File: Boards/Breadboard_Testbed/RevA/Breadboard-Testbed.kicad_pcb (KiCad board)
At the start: 2 copper layers, 85 x 56 mm, 12 parts, among them J1 main_conn_10, J10 Arduino-right, J12 Conn_02x12_Counter_Clockwise, J2 main_conn_12, J3 Conn_02x14_Odd_Even, J4 Conn_02x14_Odd_Even, J5 Conn_02x10_Counter_Clockwise, J6 Conn_02x14_Odd_Even, J7 Arduino-left, J8 Conn_02x10_Counter_Clockwise, J9 Conn_02x12_Counter_Clockwise

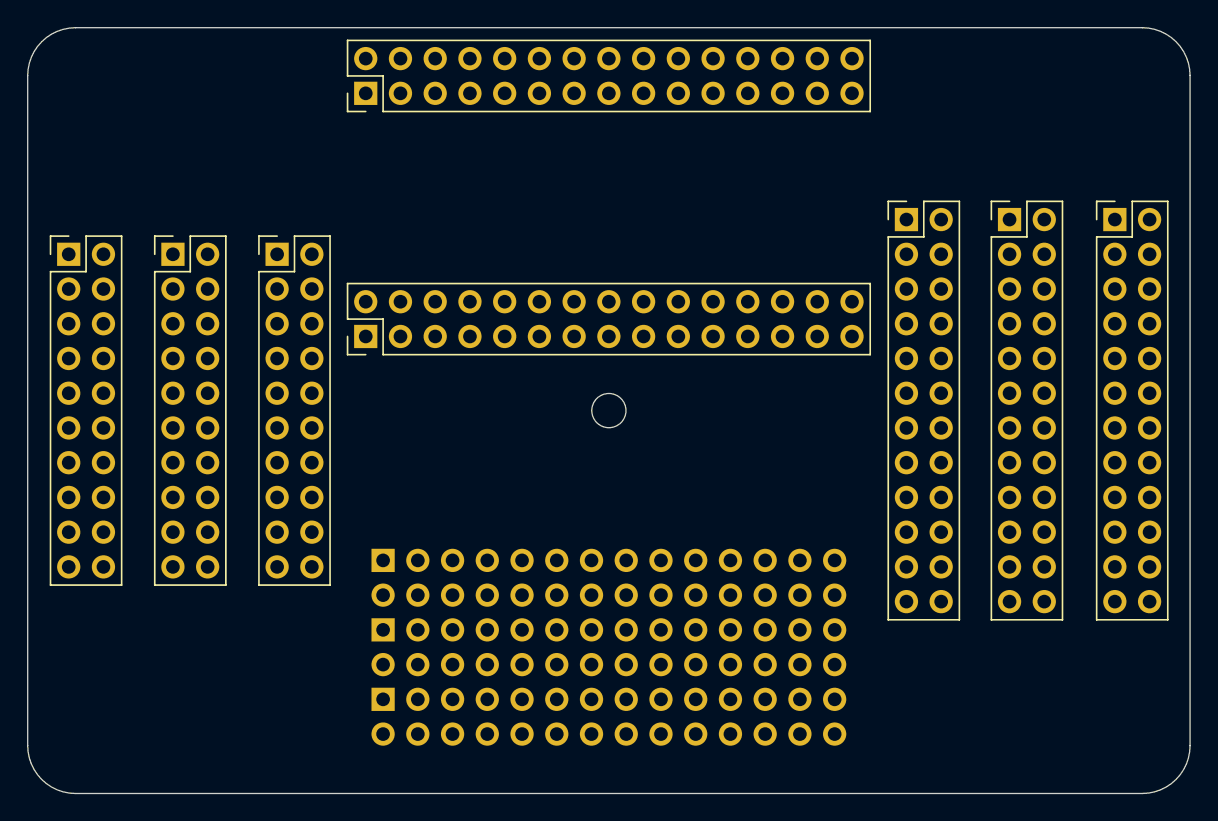
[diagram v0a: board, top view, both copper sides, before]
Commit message: Routing Complete  Test-RevA board
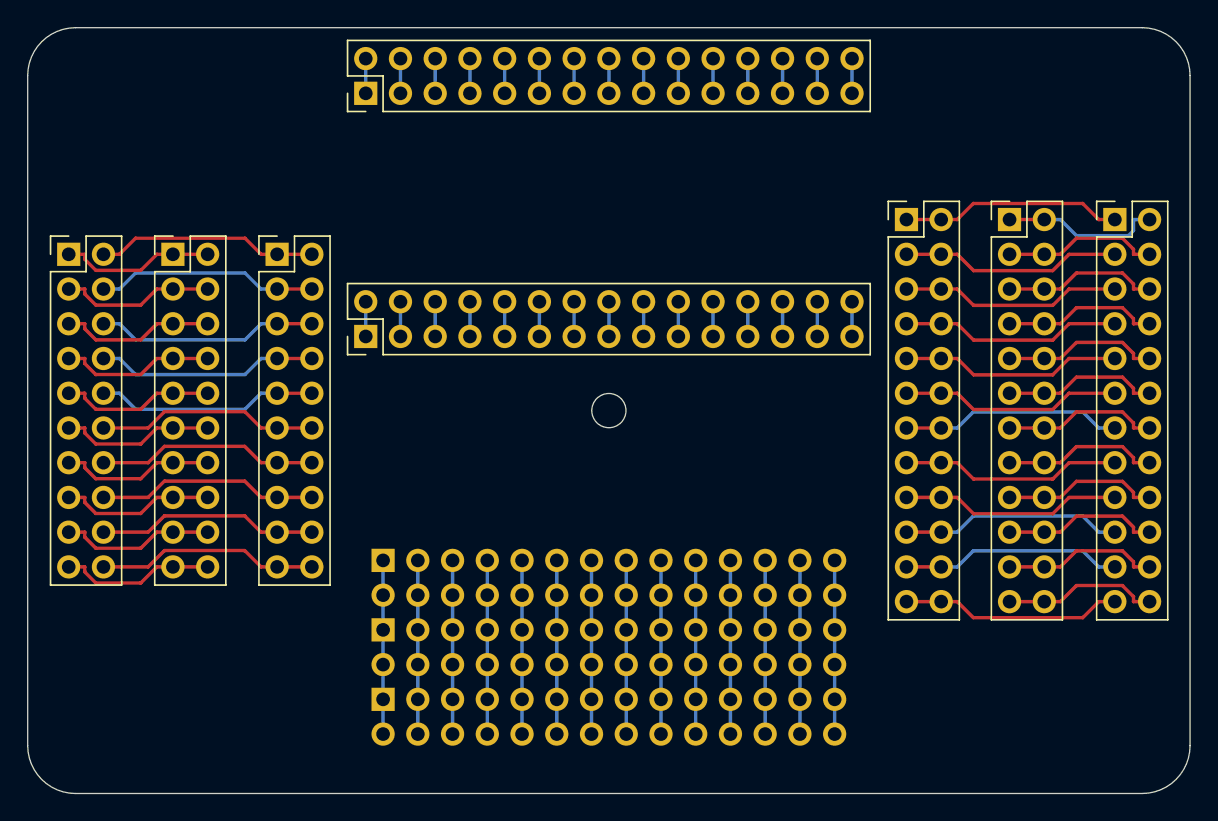
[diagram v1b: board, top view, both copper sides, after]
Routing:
- net Net-(J2-Pad9): track 0.00 -> 16.2 mm
- net Net-(J2-Pad5): track 0.00 -> 16.2 mm
- net Net-(J2-Pad3): track 0.00 -> 16.2 mm
- net Net-(J2-Pad17): track 0.00 -> 16.2 mm
- net Net-(J2-Pad15): track 0.00 -> 16.2 mm
- net Net-(J2-Pad11): track 0.00 -> 16.2 mm
- net Net-(J1-Pad20): track 0.00 -> 16.2 mm
- net Net-(J1-Pad18): track 0.00 -> 16.2 mm
- net Net-(J1-Pad14): track 0.00 -> 16.2 mm
- net Net-(J1-Pad12): track 0.00 -> 16.2 mm
- net Net-(J2-Pad7): track 0.00 -> 16.2 mm
- net Net-(J1-Pad16): track 0.00 -> 16.2 mm
- net Net-(J2-Pad23): track 0.00 -> 16.2 mm
- net Net-(J2-Pad21): track 0.00 -> 16.2 mm
- net Net-(J2-Pad19): track 0.00 -> 16.2 mm
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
